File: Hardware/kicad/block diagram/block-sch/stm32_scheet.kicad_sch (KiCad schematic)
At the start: 25 parts, among them J3 USB_A, J4 Conn_01x03, J5 Conn_02x02_Counter_Clockwise, Q2 BC817, SW1 NRST_BUTT, U16 CS43L21, U17 CAT24C256, U18 USBLC6-4SC6, U6 STM32L4Q5, Y1 Crystal

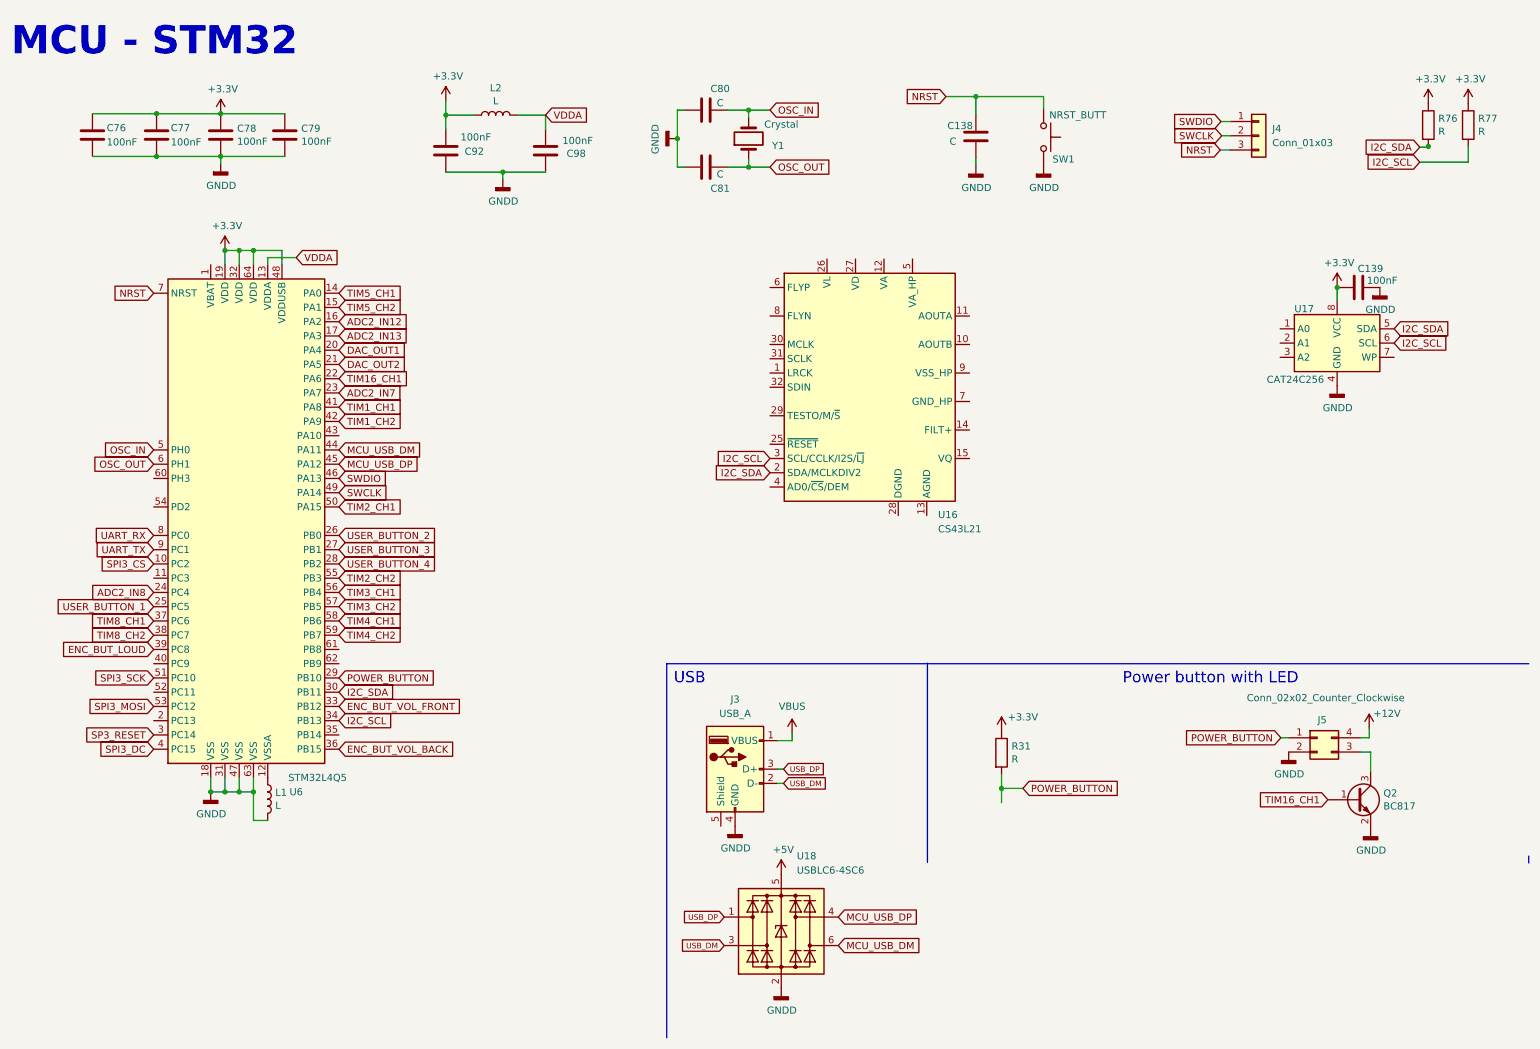
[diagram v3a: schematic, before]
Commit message: new
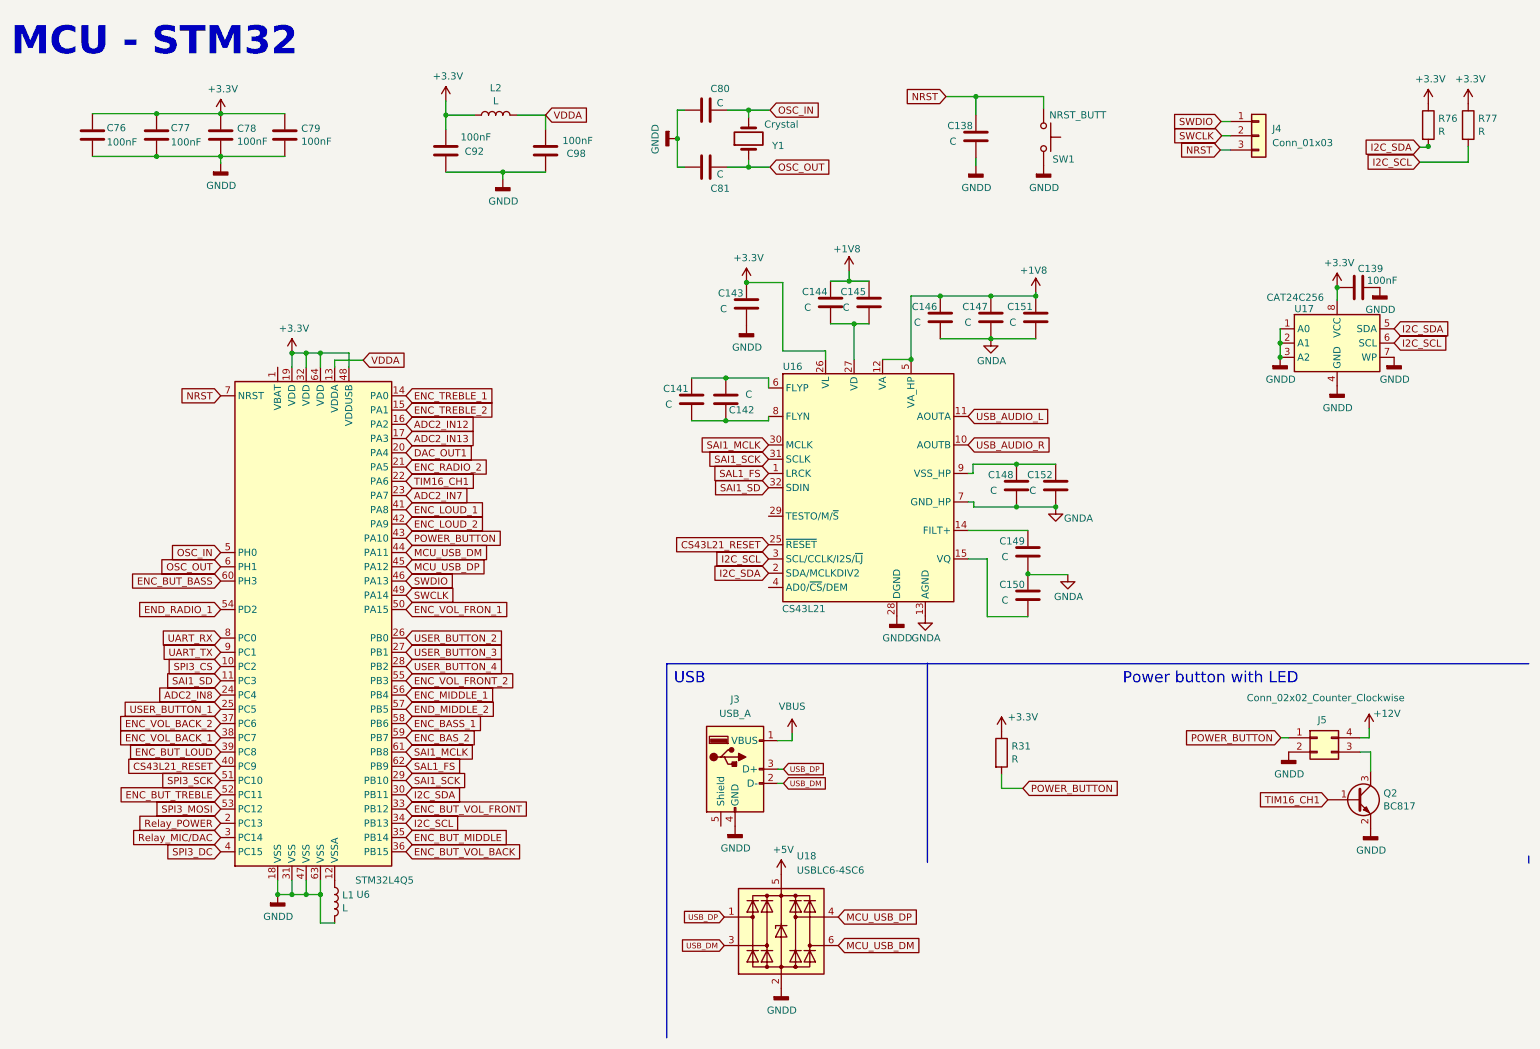
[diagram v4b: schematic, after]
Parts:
- added C141, C142: C, Capacitor_SMD:C_1206_3216Metric, symbol Device:C
- added C143, C144, C145, C146, C147, C148, C149, C150, C151, C152: C, Capacitor_SMD:C_0805_2012Metric, symbol Device:C
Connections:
- net +3V3: now also U16.26 (VL), C143.1
- net GNDD: now also U16.28 (DGND), U17.1 (A0), U17.2 (A1), U17.3 (A2), U17.7 (WP), C143.2
- net POWER_BUTTON: now also U6.43 (PA10); no longer U6.29 (PB10)
- net SAI1_SD: now reaches U6.11 (PC3)
- net SAI1_SD: now also U16.32 (SDIN)
- net Relay_POWER: now reaches U6.2 (PC13)
- net ENC_BUT_MIDDLE: now reaches U6.35 (PB14)
- net CS43L21_RESET: now reaches U6.40 (PC9)
- net CS43L21_RESET: now also U16.25 (~{RESET})
- net ENC_BUT_TREBLE: now reaches U6.52 (PC11)
- net END_RADIO_1: now reaches U6.54 (PD2)
- net ENC_BUT_BASS: now reaches U6.60 (PH3)
- net SAI1_MCLK: now reaches U6.61 (PB8)
- net SAI1_MCLK: now also U16.30 (MCLK)
- net SAL1_FS: now reaches U6.62 (PB9)
- net SAL1_FS: now also U16.1 (LRCK)
- net USB_AUDIO_R: now reaches U16.10 (AOUTB)
- net USB_AUDIO_L: now reaches U16.11 (AOUTA)
- net +1V8: now reaches U16.12 (VA)
- net +1V8: now also U16.5 (VA_HP), C144.1, C145.1, C146.1, C147.1, C151.1
- net GNDA: now reaches U16.13 (AGND), U16.33 (AGND)
- net GNDA: now also U16.7 (GND_HP), C146.2, C147.2, C148.2, C149.2, C150.1, C151.2, C152.2
- net at U16.14 (FILT+): now also C149.1
- net at U16.15 (VQ): now also C150.2
- net at U16.27 (VD): now also C144.2, C145.2
- net SAI1_SCK: now reaches U16.31 (SCLK)
- net SAI1_SCK: now also U6.29 (PB10)
- net at U16.6 (FLYP): now also C141.1, C142.2
- net at U16.8 (FLYN): now also C141.2, C142.1
- net at U16.9 (VSS_HP): now also C148.1, C152.1
- net DAC_OUT2 renamed ENC_RADIO_2
- net SP3_RESET renamed Relay_MIC/DAC
- net TIM1_CH1 renamed ENC_LOUD_1
- net TIM1_CH2 renamed ENC_LOUD_2
- net TIM2_CH1 renamed ENC_VOL_FRON_1
- net TIM2_CH2 renamed ENC_VOL_FRONT_2
- net TIM3_CH1 renamed ENC_MIDDLE_1
- net TIM3_CH2 renamed END_MIDDLE_2
- net TIM4_CH1 renamed ENC_BASS_1
- net TIM4_CH2 renamed ENC_BAS_2
- net TIM5_CH1 renamed ENC_TREBLE_1
- net TIM5_CH2 renamed ENC_TREBLE_2
- net TIM8_CH1 renamed ENC_VOL_BACK_2
- net TIM8_CH2 renamed ENC_VOL_BACK_1
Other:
- moved on the sheet: L1, U16, U6

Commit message: new
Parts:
- J5: footprint Connector_PinHeader_2.54mm:PinHeader_2x02_P2.54mm_Vertical -> Connector_PinSocket_1.27mm:PinSocket_2x02_P1.27mm_Vertical
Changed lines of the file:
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@@
     (property "Reference" "J5" (id 0) (at 247.65 140.843 0))
     (property "Value" "Conn_02x02_Counter_Clockwise" (id 1) (at 248.285 136.906 0))
-    (property "Footprint" "Connector_PinHeader_2.54mm:PinHeader_2x02_P2.54mm_Vertical" (id 2) (at 246.761 144.018 0)
+    (property "Footprint" "Connector_PinSocket_1.27mm:PinSocket_2x02_P1.27mm_Vertical" (id 2) (at 246.761 144.018 0)
       (effects (font (size 1.27 1.27)) hide)
     )
